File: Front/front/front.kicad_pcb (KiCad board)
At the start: 2 copper layers, 28.5 x 51.8 mm, 13 parts, among them J1 JST PH 1mm 4-Pin Connector, J2 Conn_01x10_Male, SW1 SW_Push, U1 L293D

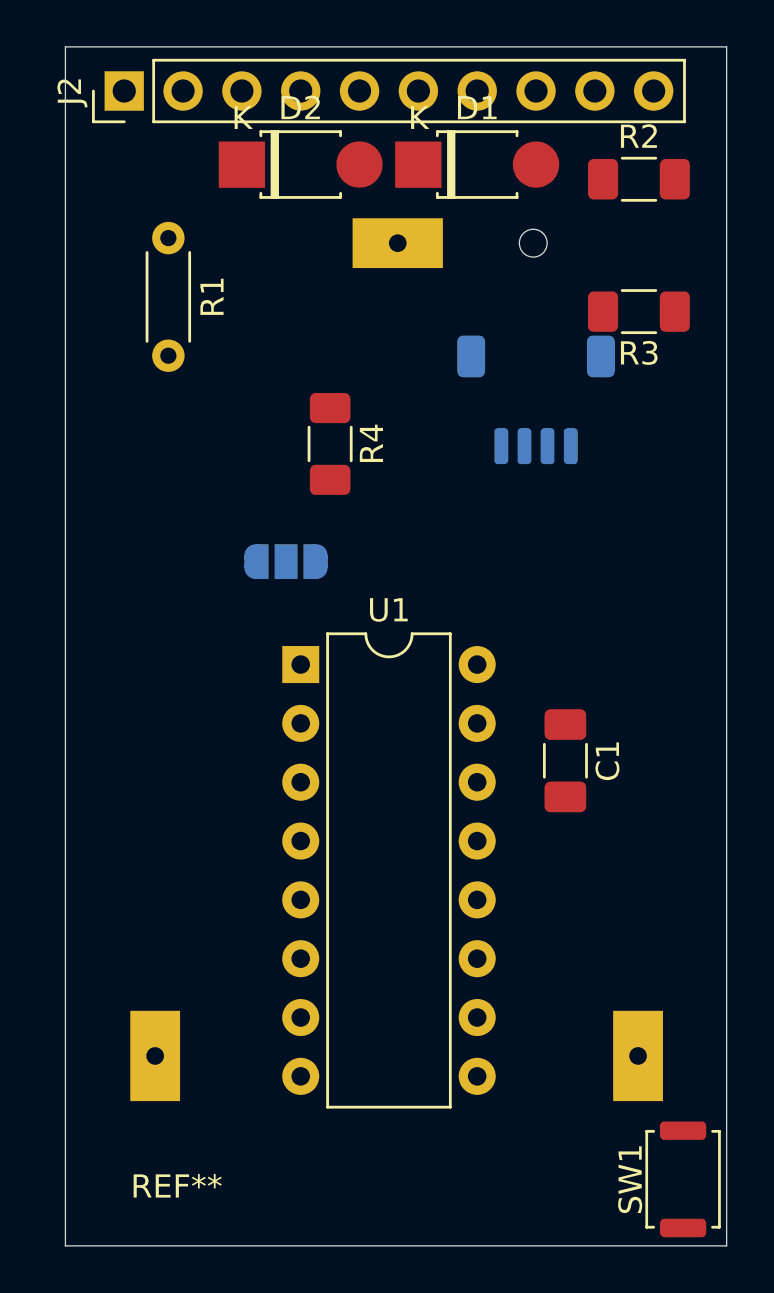
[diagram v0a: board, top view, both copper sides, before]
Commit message: Version 0.1.2 - First draft of front PCB complete
Signed-off-by: ray33ee <30669752+ray33ee@users.noreply.github.com>
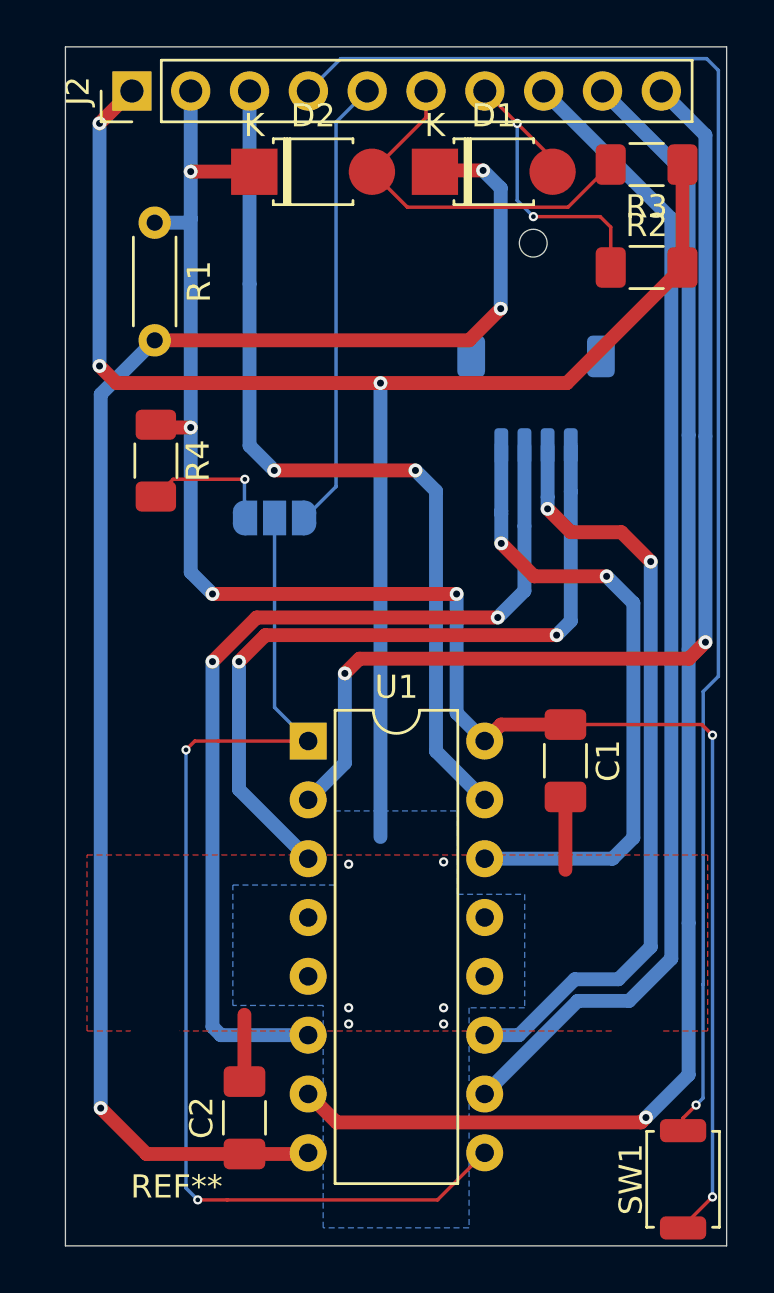
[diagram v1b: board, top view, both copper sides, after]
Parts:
- added C2: 100nF, Capacitor_SMD:C_1206_3216Metric_Pad1.33x1.80mm_HandSolder, F.Cu at (199.5, 126.2)
- J1: value JST PH 1mm 4-Pin Connector -> JST 1mm Connector
- moved R4 7.56 mm to (195.7, 97.9)
- moved R3 6.36 mm to (216.9, 85.1)
- moved R2 3.82 mm to (216.9, 89.5)
- moved U1 3.32 mm to (202.3, 110.0)
- moved JP1 1.95 mm to (200.8, 100.3)
- moved R1 0.89 mm to (195.6, 87.6)
- moved D1 0.78 mm to (207.7, 85.4)
- moved D2 0.62 mm to (199.9, 85.4)
- moved J2 0.33 mm to (194.6, 81.9)
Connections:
- net Net-(D1-Pad1) renamed /Motor_Supply_Pre
- net Net-(J1-Pad1) renamed /JST_PIN_1
- net Net-(J1-Pad2) renamed /JST_PIN_2
- net Net-(J1-Pad3) renamed /JST_PIN_3
- net Net-(J1-Pad4) renamed /JST_PIN_4
- J2 pad 5: /Enable -> /Enable_Controlled
- JP1 pad 1: /Enable -> /Enable_High
- JP1 pad 2: Net-(JP1-Pad2) -> /Enable
- JP1 pad 3: Net-(JP1-Pad3) -> /Enable_Controlled
- R4 pad 2: Net-(JP1-Pad3) -> /Enable_High
- U1 pad 1: Net-(JP1-Pad2) -> /Enable
- U1 pad 9: Net-(JP1-Pad2) -> /Enable
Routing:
- net +5V: track 0.00 -> 77.6 mm, vias 0 -> 6
- net GND: track 0.00 -> 70.1 mm, vias 0 -> 9
- net /Motor_Supply_Pre: track 0.00 -> 67.8 mm, vias 0 -> 3
- net /PushButton1: track 0.00 -> 64.9 mm, vias 0 -> 1
- net /Coil_A2: track 0.00 -> 61.8 mm, vias 0 -> 1
- net /Coil_B1: track 0.00 -> 50.2 mm
- net /Enable: track 0.00 -> 48.8 mm, vias 0 -> 2
- net /Coil_A1: track 0.00 -> 46.8 mm, vias 0 -> 2
- net /JST_PIN_2: track 0.00 -> 41.0 mm, vias 0 -> 2
- net /Coil_B2: track 0.00 -> 38.4 mm, vias 0 -> 2
- net /JST_PIN_3: track 0.00 -> 33.5 mm, vias 0 -> 2
- net /JST_PIN_4: track 0.00 -> 32.3 mm, vias 0 -> 2
- net /JST_PIN_1: track 0.00 -> 27.9 mm, vias 0 -> 2
- net /Enable_Controlled: track 0.00 -> 19.6 mm
- net /Diff_P1: track 0.00 -> 16.8 mm
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- added copper zone on B.Cu, net GND
- added copper zone on F.Cu, net GND
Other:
- net class Default: clearance 0.2 -> 0.127; trace_width 0.25 -> 0.15; via_dia 0.8 -> 0.4; via_drill 0.4 -> 0.2
- net class High Current added: clearance 0.15, trace_width 0.6, via_dia 0.6, via_drill 0.3
- rule trace_clearance: 0.2 -> 0.127
- rule trace_min: 0.2 -> 0.127
- rule via_min_drill: 0.3 -> 0.2
